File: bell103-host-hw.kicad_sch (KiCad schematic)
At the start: 6 parts, among them J2 Conn_01x02_Pin, J8 Conn_01x02

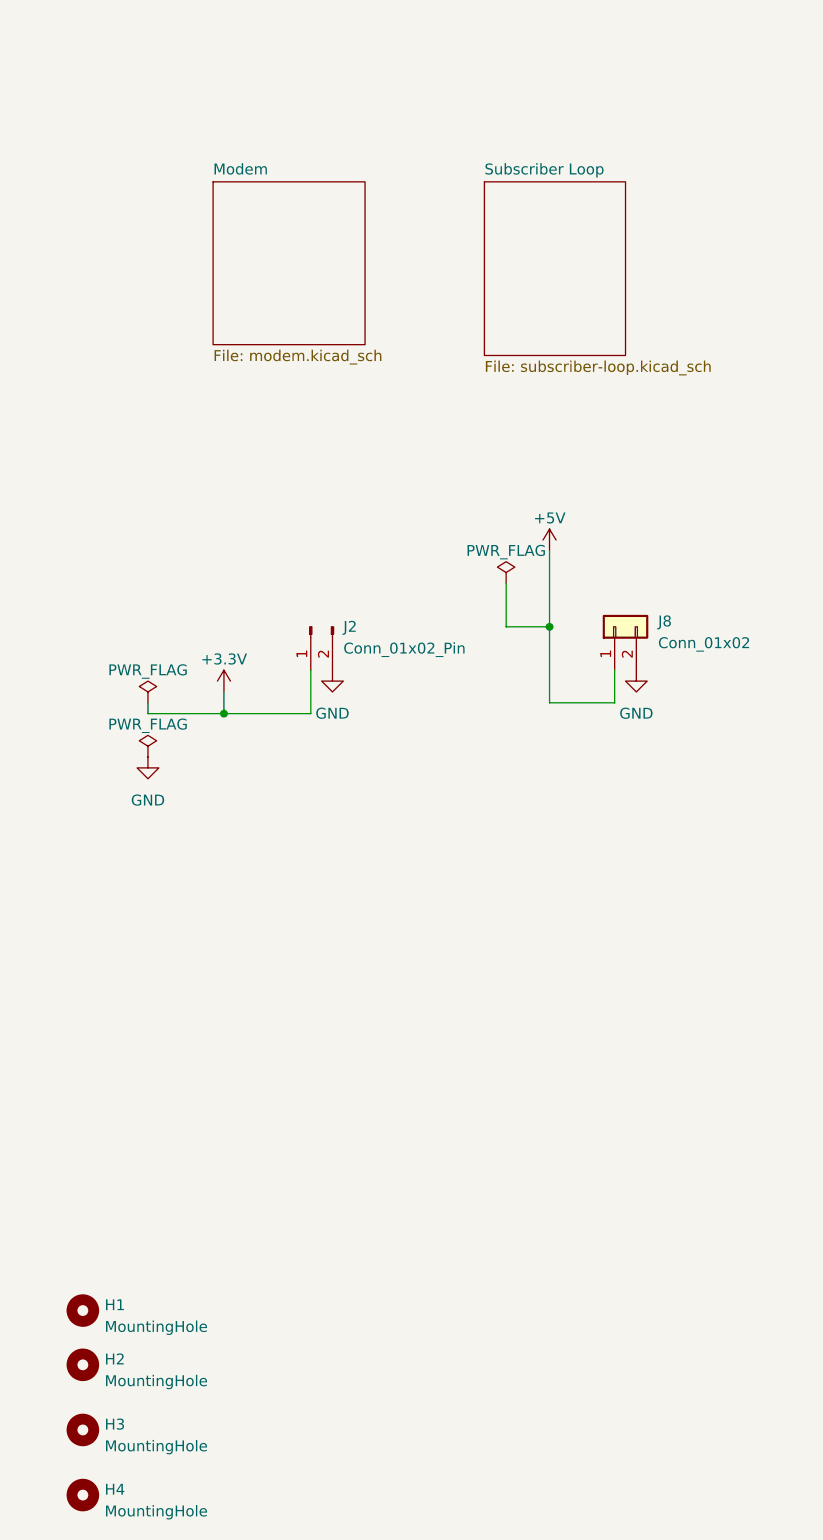
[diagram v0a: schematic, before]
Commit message: Improved docs
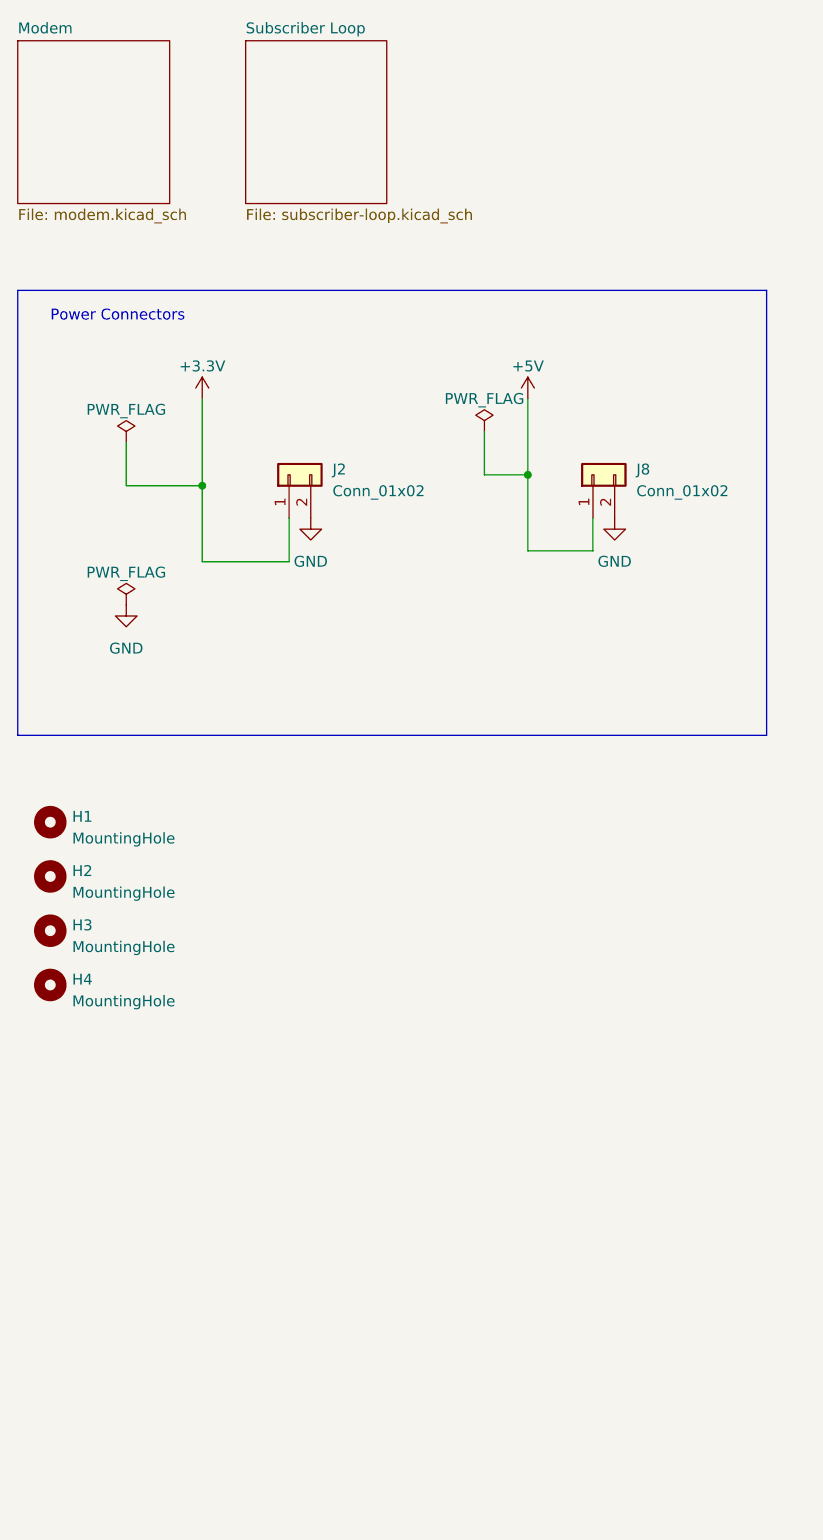
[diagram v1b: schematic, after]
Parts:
- removed J2: Conn_01x02_Pin, Connector_PinHeader_2.54mm:PinHeader_1x02_P2.54mm_Vertical, symbol Connector:Conn_01x02_Pin
- added J2: Conn_01x02, symbol Connector_Generic:Conn_01x02
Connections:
- net +3.3V: now also J2.1 (Pin_1)
- net GND: now also J2.2 (Pin_2)
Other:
- note added: "Power Connectors"
- moved on the sheet: H1, H2, H3, H4, J8
